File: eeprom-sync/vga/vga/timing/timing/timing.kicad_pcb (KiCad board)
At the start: 2 copper layers, 63.5 x 41.3 mm, 12 parts, among them J1 Conn_01x02_Male, J2 Conn_01x02_Female, J3 Conn_01x08_Female, U1 74LS161, U2 74LS161, U3 28C256, U4 74LS161, U5 74HCT574, U6 74LS161, U7 74LS08, U8 74LS161, X1 CXO_DIP8

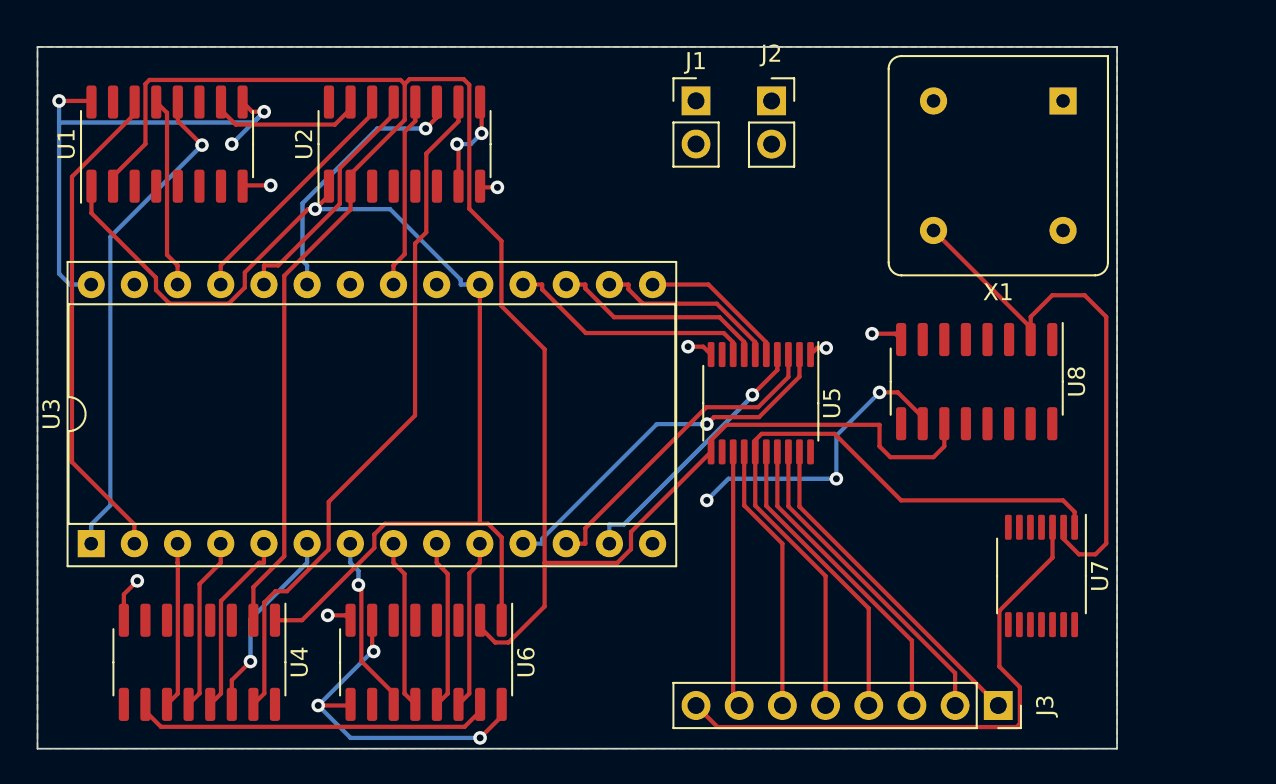
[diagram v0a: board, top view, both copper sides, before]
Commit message: final board
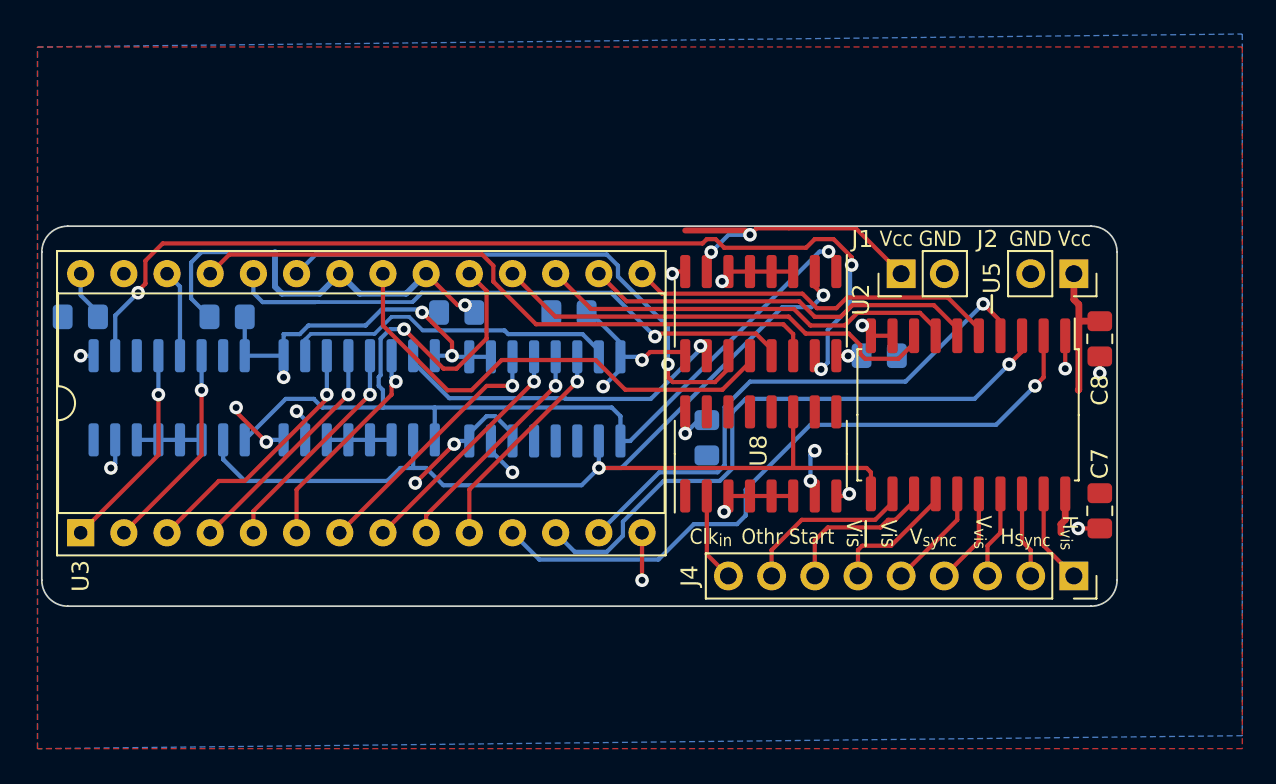
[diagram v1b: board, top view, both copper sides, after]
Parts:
- removed J3: Conn_01x08_Female, Connector_PinSocket_2.54mm:PinSocket_1x08_P2.54mm_Vertical
- removed U7: 74LS08, Package_SO:TSSOP-14_4.4x5mm_P0.65mm
- removed X1: CXO_DIP8, Oscillator:Oscillator_DIP-8
- added C1: C_Small, Capacitor_SMD:C_0805_2012Metric_Pad1.18x1.45mm_HandSolder, B.Cu at (74.7, 38.1)
- added C2: C_Small, Capacitor_SMD:C_0805_2012Metric_Pad1.18x1.45mm_HandSolder, B.Cu at (113.0, 40.4)
- added C3: C_Small, Capacitor_SMD:C_0805_2012Metric_Pad1.18x1.45mm_HandSolder, B.Cu at (88.2, 37.8)
- added C4: C_Small, Capacitor_SMD:C_0805_2012Metric_Pad1.18x1.45mm_HandSolder, B.Cu at (94.8, 37.8)
- added C5: C_Small, Capacitor_SMD:C_0805_2012Metric_Pad1.18x1.45mm_HandSolder, B.Cu at (102.9, 45.2)
- added C6: C_Small, Capacitor_SMD:C_0805_2012Metric_Pad1.18x1.45mm_HandSolder, B.Cu at (66.0, 38.1)
- added C7: C_Small, Capacitor_SMD:C_0805_2012Metric_Pad1.18x1.45mm_HandSolder, F.Cu at (126.0, 49.5)
- added C8: C_Small, Capacitor_SMD:C_0805_2012Metric_Pad1.18x1.45mm_HandSolder, F.Cu at (126.0, 39.4)
- added J4: Conn_01x09_Socket, Connector_PinSocket_2.54mm:PinSocket_1x09_P2.54mm_Vertical, F.Cu at (124.5, 53.3)
- U1, U4, U6: moved to B.Cu
- U5: footprint Package_SO:TSSOP-20_4.4x6.5mm_P0.65mm -> Package_SO:SOIC-20W_7.5x12.8mm_P1.27mm
- moved U2 23.2 mm to (106.0, 37.9), turned to -90 degrees
- moved J2 20.5 mm to (124.5, 35.6), turned to -90 degrees
- moved U4 18.2 mm to (82.4, 42.9), turned to 90 degrees
- moved U6 17.0 mm to (93.3, 42.9), turned to 90 degrees
- moved J1 15.8 mm to (114.3, 35.6), turned to 90 degrees
- moved U1 14.9 mm to (71.2, 42.9)
- moved U8 13.4 mm to (106.0, 46.2), turned to 90 degrees
- moved U5 12.2 mm to (118.2, 43.9)
- moved U3 0.89 mm to (66.0, 50.8)
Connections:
- U1 pad 3: unconnected-(U1-Pad3) -> GND
- U1 pad 4: unconnected-(U1-Pad4) -> GND
- U1 pad 5: unconnected-(U1-Pad5) -> GND
- U1 pad 6: unconnected-(U1-Pad6) -> GND
- U2 pad 3: unconnected-(U2-Pad3) -> GND
- U2 pad 4: unconnected-(U2-Pad4) -> GND
- U2 pad 5: unconnected-(U2-Pad5) -> GND
- U2 pad 6: unconnected-(U2-Pad6) -> GND
- U4 pad 3: unconnected-(U4-Pad3) -> GND
- U4 pad 4: unconnected-(U4-Pad4) -> GND
- U4 pad 5: unconnected-(U4-Pad5) -> GND
- U4 pad 6: unconnected-(U4-Pad6) -> GND
- U5 pad 12: unconnected-(U5-Pad12) -> /Othr
- U5 pad 9: unconnected-(U5-Pad9) -> GND
- U6 pad 3: unconnected-(U6-Pad3) -> GND
- U6 pad 4: unconnected-(U6-Pad4) -> GND
- U6 pad 5: unconnected-(U6-Pad5) -> GND
- U6 pad 6: unconnected-(U6-Pad6) -> GND
- U8 pad 2: Net-(U7-Pad2) -> /Clk_{in}
- U8 pad 3: unconnected-(U8-Pad3) -> GND
- U8 pad 4: unconnected-(U8-Pad4) -> GND
- U8 pad 5: unconnected-(U8-Pad5) -> GND
- U8 pad 6: unconnected-(U8-Pad6) -> GND
- U8 pad 9: unconnected-(U8-Pad9) -> VCC
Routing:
- net /CLK_{sync}: track 130.5 -> 67.9 mm, vias 0 -> 2
- net GND: track 11.3 -> 65.0 mm, vias 7 -> 14
- net Net-(U1-CET): track 9.22 -> 57.5 mm, vias 0 -> 3
- net /Clk_{pixel}: track 33.0 -> 0.00 mm
- net /Vis: track 39.1 -> 6.19 mm
- net Net-(U7-Pad2): track 32.8 -> 0.00 mm
- net /A8: track 14.4 -> 38.5 mm
- net Net-(U2-CET): track 40.8 -> 20.3 mm, vias 0 -> 1
- net /A9: track 14.4 -> 34.0 mm, vias 0 -> 1
- net Net-(U3-D0): track 21.8 -> 39.7 mm
- net /A10: track 11.3 -> 28.7 mm
- net Net-(U3-D1): track 19.0 -> 36.1 mm, vias 0 -> 1
- net /A14: track 29.3 -> 12.3 mm
- net Net-(U3-D2): track 15.7 -> 32.5 mm
- net /A12: track 29.0 -> 12.3 mm, vias 0 -> 1
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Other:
- board size 63.5 x 41.3 mm -> 63.2 x 22.4 mm
- board text added: "Clk_{in}"
- board text added: "GND Vcc"
- board text added: "H_{Sync}"
- board text added: "H_{vis}"
- board text added: "Othr"
- board text added: "Start"
- board text added: "V_{sync}"
- board text added: "V_{vis}"
- board text added: "Vcc GND"
- board text added: "Vis"
- board text added: "~{Vis}"
